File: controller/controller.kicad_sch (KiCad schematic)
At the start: 7 parts, among them IC1 TCST2103, J1 Screw_Terminal_01x08, U1 74HC590

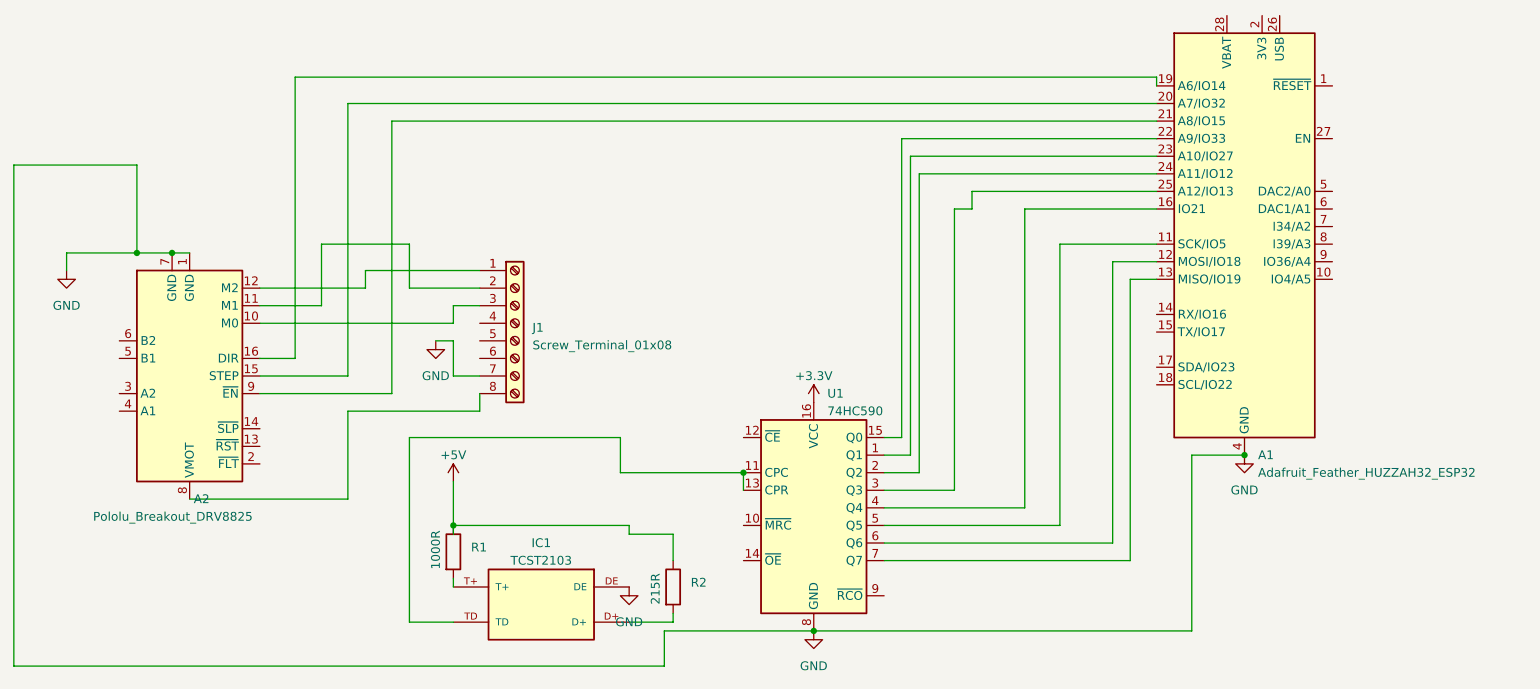
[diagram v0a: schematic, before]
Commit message: recent changes
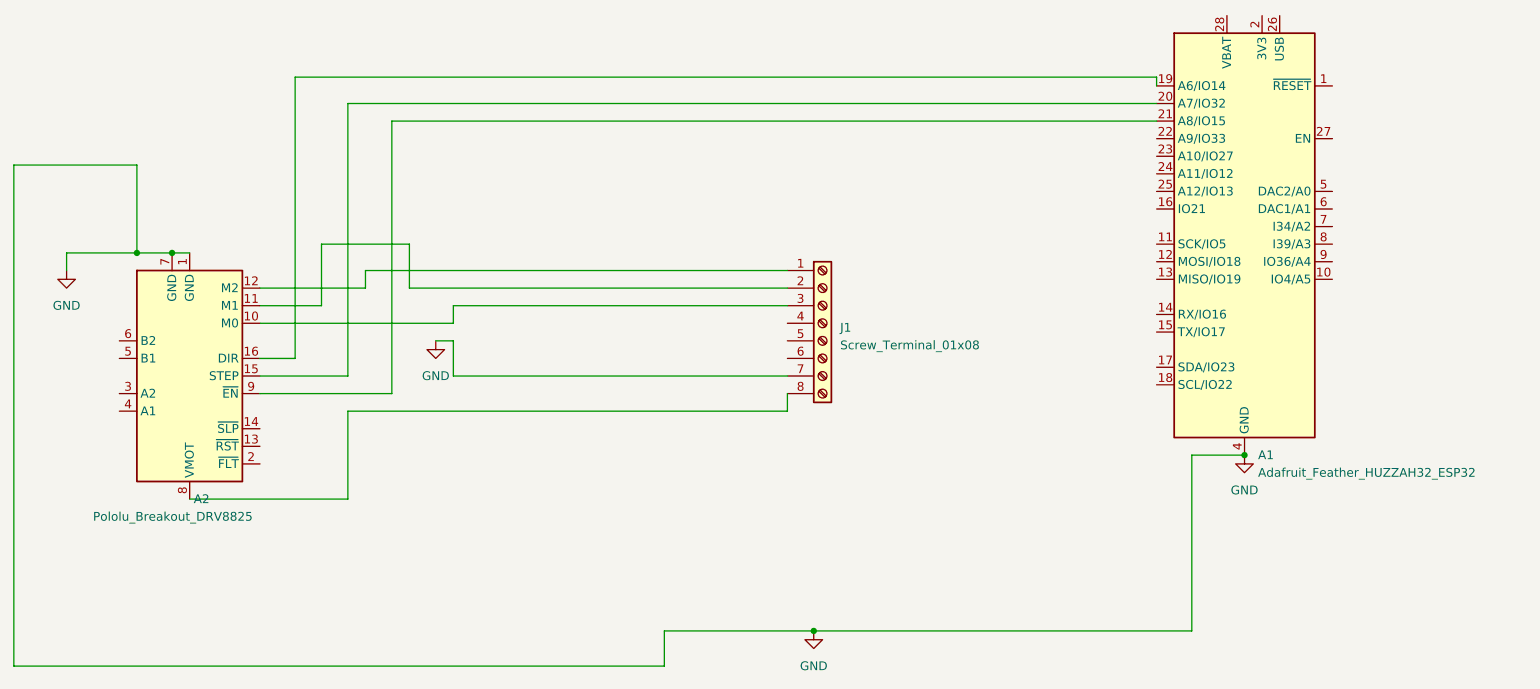
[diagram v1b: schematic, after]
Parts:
- removed IC1: TCST2103, TCST2103:TCST2103, symbol TCST2103:TCST2103
- removed R1: 1000R, Resistor_THT:R_Axial_DIN0309_L9.0mm_D3.2mm_P12.70mm_Horizontal, symbol Device:R
- removed R2: 215R, Resistor_THT:R_Axial_DIN0309_L9.0mm_D3.2mm_P12.70mm_Horizontal, symbol Device:R
- removed U1: 74HC590, Package_DIP:DIP-16_W7.62mm_LongPads, symbol 74xx:74HC590
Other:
- moved on the sheet: J1
